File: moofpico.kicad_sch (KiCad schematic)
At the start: 21 parts, among them J1 Conn_01x04, J100 Bus_Apple_II_Card_Side, J2 Micro_SD_Card_Det2, Q1 BS170, SW1 SW_DIP_x02, U2 74F11, U3 74LVC245, U4 74LVC245, U5 74LVC245, U6 RaspberryPi_Pico

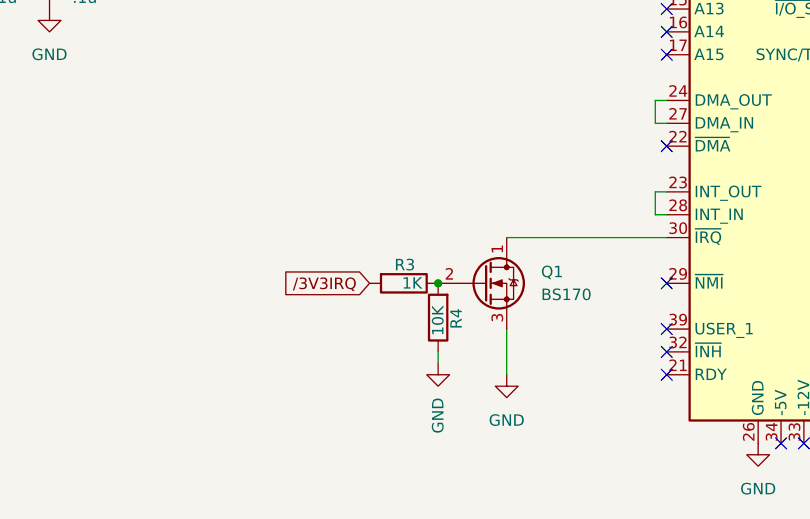
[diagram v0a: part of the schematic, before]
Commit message: more faffing about with moving components
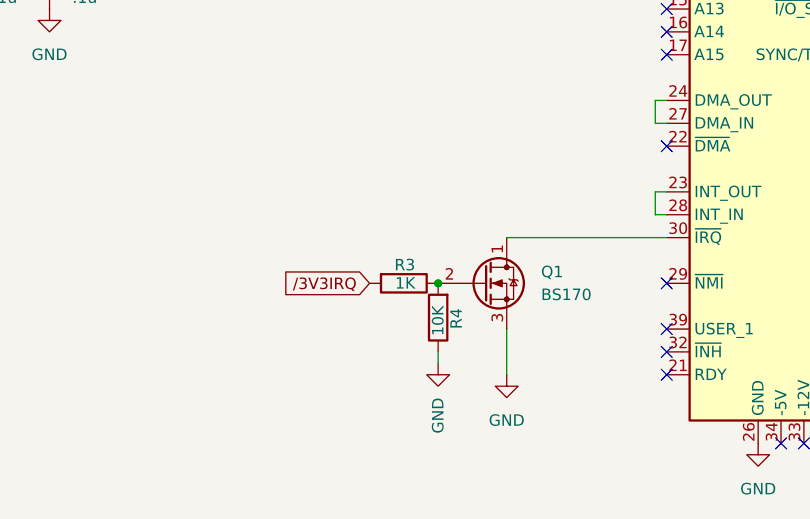
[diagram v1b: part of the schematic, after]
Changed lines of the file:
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@@
 		)
 		(property "Value" "1K"
-			(at 92.202 172.72 90)
+			(at 91.44 172.72 90)
 			(effects
 				(font
